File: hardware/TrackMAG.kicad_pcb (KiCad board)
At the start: 4 copper layers, 36 x 36 mm, 58 parts, among them J1 USB_C_Socket_USB2.0, J2 Conn_Debug, SW1 SW_RESET, SW2 SW_BOOT, SW3 SW_CALIBRATE, U1 LSM6DS3TR-C, U2 USBLC6-2P6, U3 STM32F103C8T6, U4 LIS2MDL, U5 AMS1117-3.3, Y1 16MHz

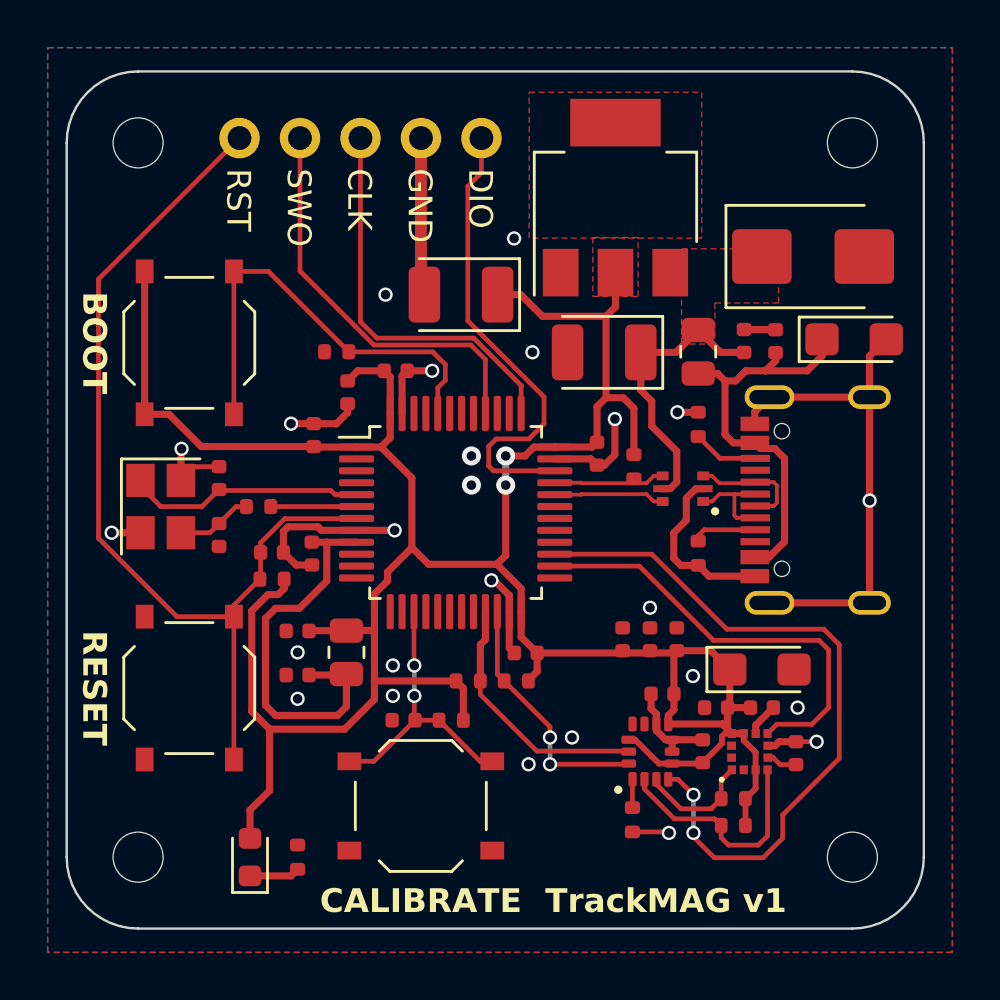
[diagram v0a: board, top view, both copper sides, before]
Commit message: Cleanup
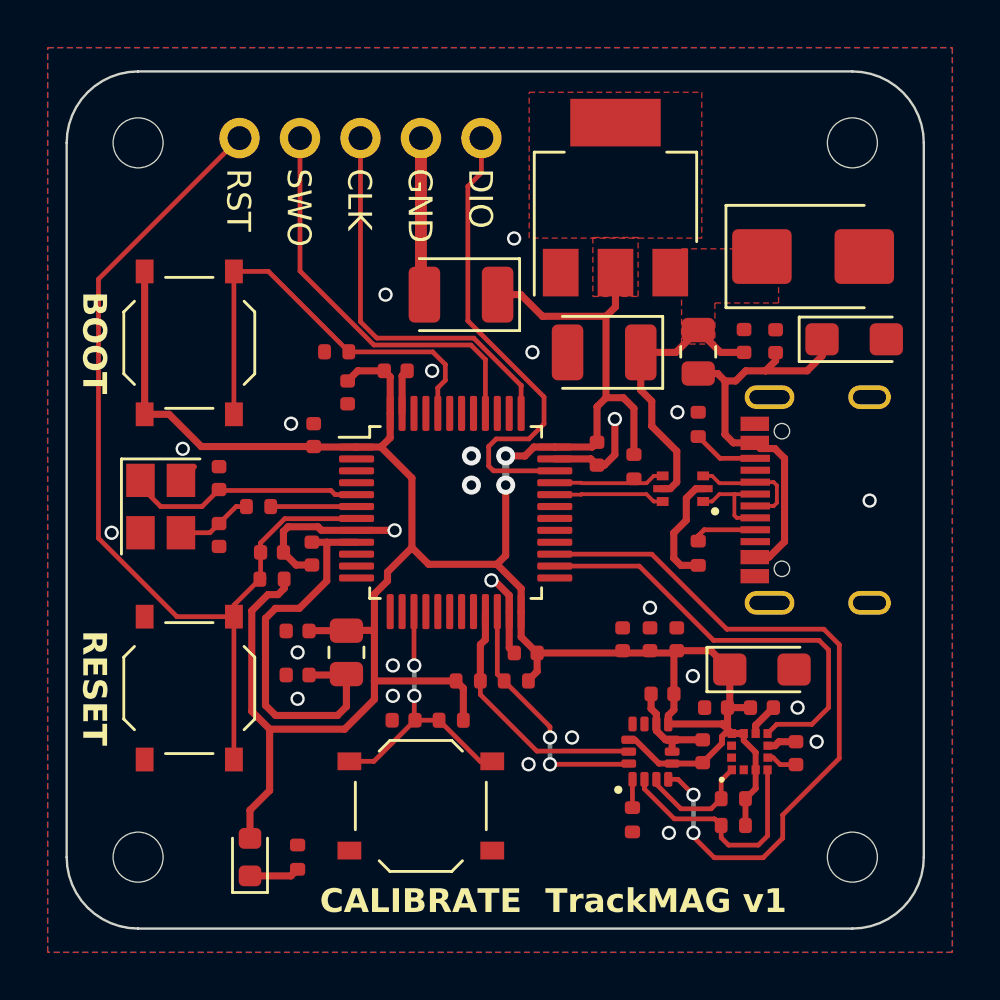
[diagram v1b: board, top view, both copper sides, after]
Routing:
- net GND: track 72.8 -> 37.1 mm
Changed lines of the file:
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@@
   (segment (start 146.3 90.375) (end 146.3 91.45) (width 0.3) (layer "F.Cu") (net 2))
   (segment (start 130.1 90.125) (end 129.9 90.325) (width 0.3) (layer "F.Cu") (net 2))
-  (segment (start 154.52 84.68) (end 154.52 82.955) (width 0.3) (layer "F.Cu") (net 2))
-  (segment (start 127.2 87.6) (end 126.175 87.6) (width 0.2) (layer "F.Cu") (net 2))
   (segment (start 134.8875 85.3625) (end 134.8875 83.7875) (width 0.3) (layer "F.Cu") (net 2))
-  (segment (start 132.12 85.795) (end 131.175 85.795) (width 0.3) (layer "F.Cu") (net 2))
   (segment (start 150.25 99.32) (end 150.55 99.32) (width 0.3) (layer "F.Cu") (net 2))
   (segment (start 146.3 91.45) (end 146.595 91.745) (width 0.3) (layer "F.Cu") (net 2))
-  (segment (start 154.52 84.68) (end 154.52 89.02) (width 0.3) (layer "F.Cu") (net 2))
-  (segment (start 149.7 85.8) (end 149.7 85.3) (width 0.3) (layer "F.Cu") (net 2))
   (segment (start 141.3 87.275) (end 142.815 87.275) (width 0.3) (layer "F.Cu") (net 2))
-  (segment (start 150.32 93.32) (end 154.52 93.32) (width 0.3) (layer "F.Cu") (net 2))
-  (segment (start 122.69 90.375) (end 123.9 90.375) (width 0.3) (layer "F.Cu") (net 2))
   (segment (start 149.7375 98.4625) (end 149.7375 98.8075) (width 0.3) (layer "F.Cu") (net 2))
   (segment (start 139.3875 93.004523) (end 138.756292 92.373315) (width 0.3) (layer "F.Cu") (net 2))
@@
   (segment (start 125.59 88.165) (end 125.6 88.175) (width 0.2) (layer "F.Cu") (net 2))
   (segment (start 131.1 91.73) (end 130.435 91.73) (width 0.3) (layer "F.Cu") (net 2))
-  (segment (start 150.32 84.68) (end 154.52 84.68) (width 0.3) (layer "F.Cu") (net 2))
-  (segment (start 125.6 86.875) (end 125.625 86.85) (width 0.2) (layer "F.Cu") (net 2))
-  (segment (start 132.125 85.8) (end 132.12 85.795) (width 0.3) (layer "F.Cu") (net 2))
   (segment (start 129.905 90.33) (end 129.905 91.2) (width 0.3) (layer "F.Cu") (net 2))
   (segment (start 151.2625 99.32) (end 151.43 99.1525) (width 0.2) (layer "F.Cu") (net 2))
-  (segment (start 152.3 99.1525) (end 151.43 99.1525) (width 0.2) (layer "F.Cu") (net 2))
   (segment (start 146.23 99.07) (end 147.51 99.07) (width 0.3) (layer "F.Cu") (net 2))
   (segment (start 139.3875 93.6875) (end 139.3875 95.2125) (width 0.3) (layer "F.Cu") (net 2))
@@
   (segment (start 150.55 99.32) (end 150.7175 99.1525) (width 0.3) (layer "F.Cu") (net 2))
   (segment (start 150.48 97.72) (end 149.7375 98.4625) (width 0.3) (layer "F.Cu") (net 2))
-  (segment (start 149.25 81.84) (end 150.565 81.84) (width 0.3) (layer "F.Cu") (net 2))
-  (segment (start 149.7 92.2) (end 147.78 92.2) (width 0.3) (layer "F.Cu") (net 2))
   (segment (start 143.825 87.1) (end 143.825 85.6) (width 0.3) (layer "F.Cu") (net 2))
-  (segment (start 146.45 85.315) (end 147.325 85.315) (width 0.3) (layer "F.Cu") (net 2))
   (segment (start 129.9 90.325) (end 129.905 90.33) (width 0.3) (layer "F.Cu") (net 2))
-  (segment (start 125.6 88.175) (end 125.6 86.875) (width 0.3) (layer "F.Cu") (net 2))
   (segment (start 154.52 89.03) (end 154.525 89.025) (width 0.3) (layer "F.Cu") (net 2))
   (segment (start 139.3875 93.6875) (end 139.3875 93.004523) (width 0.3) (layer "F.Cu") (net 2))
-  (segment (start 132.6 84.96) (end 132.6 85.325) (width 0.3) (layer "F.Cu") (net 2))
   (segment (start 139.3875 95.2125) (end 139.6 95.425) (width 0.3) (layer "F.Cu") (net 2))
-  (segment (start 144.5625 102.94) (end 146.0525 102.94) (width 0.2) (layer "F.Cu") (net 2))
-  (segment (start 149.7 85.3) (end 150.32 84.68) (width 0.3) (layer "F.Cu") (net 2))
   (segment (start 154 78.2) (end 153.75 78.45) (width 0.3) (layer "F.Cu") (net 2))
   (segment (start 132.975 90.275) (end 131.5 90.275) (width 0.3) (layer "F.Cu") (net 2))
   (segment (start 146.3 90.375) (end 146.825 89.85) (width 0.3) (layer "F.Cu") (net 2))
-  (segment (start 154.52 82.955) (end 155.225 82.25) (width 0.3) (layer "F.Cu") (net 2))
   (segment (start 131.35 90.125) (end 130.1 90.125) (width 0.3) (layer "F.Cu") (net 2))
   (segment (start 143.075 87.535) (end 143.39 87.535) (width 0.3) (layer "F.Cu") (net 2))
   (segment (start 153.75 78.675) (end 153.75 78.45) (width 0.3) (layer "F.Cu") (net 2))
-  (segment (start 147.78 92.2) (end 147.325 91.745) (width 0.3) (layer "F.Cu") (net 2))
   (segment (start 131.5 90.275) (end 131.35 90.125) (width 0.3) (layer "F.Cu") (net 2))
-  (segment (start 132.6 85.325) (end 132.125 85.8) (width 0.3) (layer "F.Cu") (net 2))
+  (segment (start 125.675 88.1) (end 125.6 88.175) (width 0.2) (layer "F.Cu") (net 2))
   (segment (start 143.39 87.535) (end 143.825 87.1) (width 0.3) (layer "F.Cu") (net 2))
   (segment (start 134.8875 83.7875) (end 135.1 83.575) (width 0.3) (layer "F.Cu") (net 2))
   (segment (start 147.51 99.07) (end 147.5125 99.0725) (width 0.3) (layer "F.Cu") (net 2))
   (segment (start 145.5675 98.4075) (end 145.5675 98.683155) (width 0.3) (layer "F.Cu") (net 2))
-  (segment (start 135.1 83.575) (end 136.15 83.575) (width 0.3) (layer "F.Cu") (net 2))
   (segment (start 146.825 89.85) (end 146.825 88.925) (width 0.3) (layer "F.Cu") (net 2))
   (segment (start 154.52 89.02) (end 154.525 89.025) (width 0.3) (layer "F.Cu") (net 2))
-  (segment (start 154.52 93.32) (end 154.52 89.03) (width 0.3) (layer "F.Cu") (net 2))
   (segment (start 146.0525 102.94) (end 146.095 102.9825) (width 0.2) (layer "F.Cu") (net 2))
-  (segment (start 130.225 85.795) (end 131.175 85.795) (width 0.3) (layer "F.Cu") (net 2))
   (segment (start 145.5675 98.4075) (end 145.5675 97.9875) (width 0.3) (layer "F.Cu") (net 2))
   (segment (start 145.954345 99.07) (end 146.23 99.07) (width 0.3) (layer "F.Cu") (net 2))
@@
   (via (at 137.8 87.15) (size 0.8) (drill 0.4) (layers "F.Cu" "B.Cu") (free) (net 2))
   (via (at 154.525 89.025) (size 0.6) (drill 0.4) (layers "F.Cu" "B.Cu") (net 2))
-  (via (at 125.625 86.85) (size 0.6) (drill 0.4) (layers "F.Cu" "B.Cu") (net 2))
+  (via (at 125.675 86.85) (size 0.6) (drill 0.4) (layers "F.Cu" "B.Cu") (net 2))
   (via (at 136.15 83.575) (size 0.6) (drill 0.4) (layers "F.Cu" "B.Cu") (net 2))
   (via (at 130.225 85.795) (size 0.6) (drill 0.4) (layers "F.Cu" "B.Cu") (net 2))
